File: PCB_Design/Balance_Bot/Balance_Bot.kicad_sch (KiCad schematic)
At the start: 29 parts, among them J1 DC Motor A, J2 DC Motor B, J3 Motor Power, Q1 BSS138, Q2 BSS138, U1 MPU-6050, U2 AP2112K-3.3, U3 DRV8871DDA, U4 DRV8871DDA

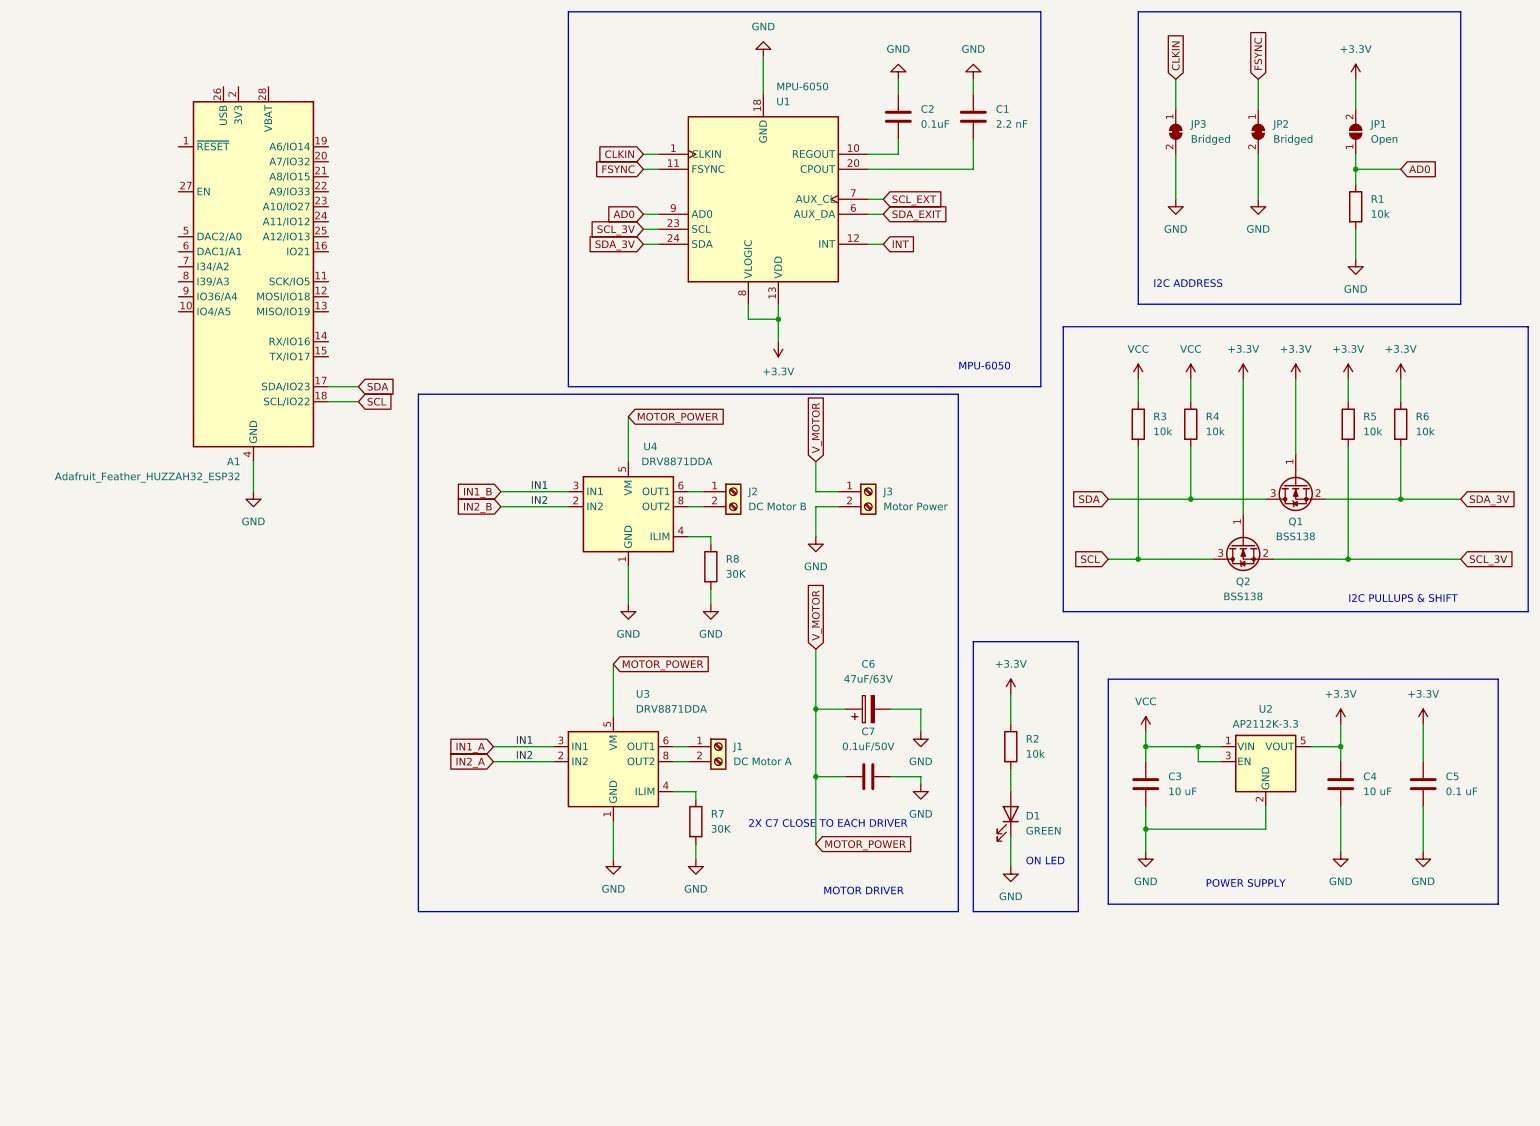
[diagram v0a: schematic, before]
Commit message: board design
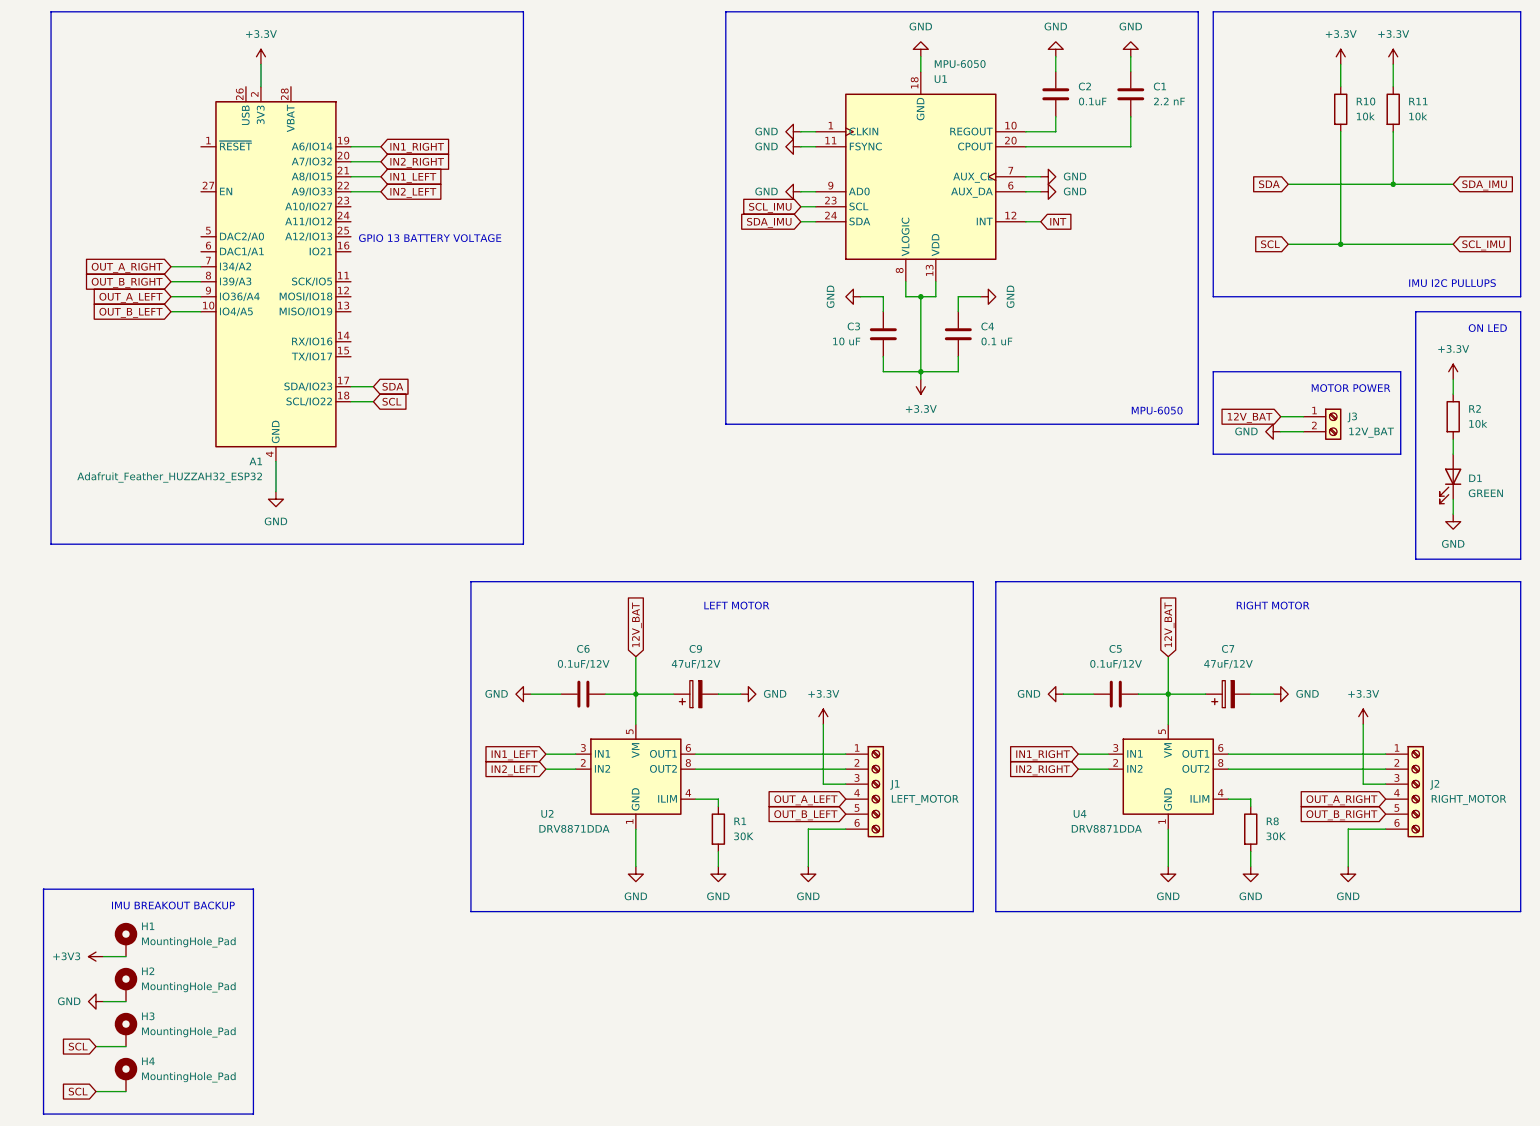
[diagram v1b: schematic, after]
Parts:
- removed C6: 47uF/63V, symbol Device:C_Polarized
- removed C7: 0.1uF/50V, Capacitor_SMD:C_0805_2012Metric, symbol Device:C
- removed J1: DC Motor A, symbol Connector:Screw_Terminal_01x02
- removed J2: DC Motor B, symbol Connector:Screw_Terminal_01x02
- removed JP1: Open, Jumper:SolderJumper-2_P1.3mm_Open_RoundedPad1.0x1.5mm, symbol Jumper:SolderJumper_2_Open
- removed JP2, JP3: Bridged, Jumper:SolderJumper-2_P1.3mm_Bridged_RoundedPad1.0x1.5mm, symbol Jumper:SolderJumper_2_Bridged
- removed Q1, Q2: BSS138, Package_TO_SOT_SMD:SOT-23, symbol Transistor_FET:BSS138
- removed R3, R4, R5, R6: 10k, Resistor_SMD:R_0805_2012Metric, symbol Device:R
- removed R7: 30K, Resistor_SMD:R_0805_2012Metric, symbol Device:R
- removed U2: AP2112K-3.3, Package_TO_SOT_SMD:SOT-23-5, symbol Regulator_Linear:AP2112K-3.3
- removed U3: DRV8871DDA, Package_SO:Texas_HTSOP-8-1EP_3.9x4.9mm_P1.27mm_EP2.95x4.9mm_Mask2.4x3.1mm_ThermalVias, symbol Driver_Motor:DRV8871DDA
- added C6: 0.1uF/12V, Capacitor_SMD:C_0805_2012Metric, symbol Device:C
- added C7, C9: 47uF/12V, symbol Device:C_Polarized
- added H1, H2, H3, H4: MountingHole_Pad, symbol Mechanical:MountingHole_Pad
- added J1: LEFT_MOTOR, TerminalBlock_Phoenix:TerminalBlock_Phoenix_PT-1,5-6-3.5-H_1x06_P3.50mm_Horizontal, symbol Connector:Screw_Terminal_01x06
- added J2: RIGHT_MOTOR, TerminalBlock_Phoenix:TerminalBlock_Phoenix_PT-1,5-6-3.5-H_1x06_P3.50mm_Horizontal, symbol Connector:Screw_Terminal_01x06
- added R10, R11: 10k, Resistor_SMD:R_0805_2012Metric, symbol Device:R
- added U2: DRV8871DDA, Package_SO:Texas_HTSOP-8-1EP_3.9x4.9mm_P1.27mm_EP2.95x4.9mm_Mask2.4x3.1mm_ThermalVias, symbol Driver_Motor:DRV8871DDA
- C4: value 10 uF -> 0.1 uF
- C5: value 0.1 uF -> 0.1uF/12V
- J3: value Motor Power -> 12V_BAT
- R1: value 10k -> 30K
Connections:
- net CLKIN is gone; now on net GND: U1.1 (CLKIN)
- net FSYNC is gone; now on net GND: U1.11 (FSYNC)
- net IN1_A is gone; now on net IN1_RIGHT: U4.3 (IN1)
- net IN2_A is gone; now on net IN2_RIGHT: U4.2 (IN2)
- net SCL_3V is gone; now on net SCL: U1.23 (SCL)
- net SCL_EXT is gone; now on net GND: U1.7 (AUX_CL)
- net SDA_3V is gone; now on net SDA: U1.24 (SDA)
- net SDA_EXIT is gone; now on net GND: U1.6 (AUX_DA)
- net VCC is gone; now on net +3.3V: C3.1
- net +3.3V: now also A1.2 (3V3), J1.3 (Pin_3), J2.3 (Pin_3), R10.1, R11.1; no longer C5.1
- net GND: now also U1.9 (AD0), C6.2, C7.2, C9.2, H2.1, J1.6 (Pin_6), J2.6 (Pin_6), U2.1 (GND), U2.7 (GND), U2.9 (GND)
- net SCL: now also H3.1, H4.1, R10.2
- net SDA: now also R11.2
- net at U4.6 (OUT1): now also J2.1 (Pin_1)
- net at U4.8 (OUT2): now also J2.2 (Pin_2)
- net OUT_B_LEFT: now reaches A1.10 (IO4/A5)
- net OUT_B_LEFT: now also J1.5 (Pin_5)
- net IN1_RIGHT: now reaches A1.19 (A6/IO14)
- net IN2_RIGHT: now reaches A1.20 (A7/IO32)
- net IN1_LEFT: now reaches A1.21 (A8/IO15)
- net IN1_LEFT: now also U2.3 (IN1)
- net IN2_LEFT: now reaches A1.22 (A9/IO33)
- net IN2_LEFT: now also U2.2 (IN2)
- net OUT_A_RIGHT: now reaches A1.7 (I34/A2)
- net OUT_A_RIGHT: now also J2.4 (Pin_4)
- net OUT_B_RIGHT: now reaches A1.8 (I39/A3)
- net OUT_B_RIGHT: now also J2.5 (Pin_5)
- net OUT_A_LEFT: now reaches A1.9 (IO36/A4)
- net OUT_A_LEFT: now also J1.4 (Pin_4)
- net AD0: no longer names the net of R1.1
- net AD0: now also U2.4 (ILIM); no longer U1.9 (AD0)
- net MOTOR_POWER renamed 12V_BAT
- net 12V_BAT: now also C5.1, C6.1, C7.1, C9.1, U2.5 (VM)
- new net: J1.1 (Pin_1), U2.6 (OUT1)
- new net: J1.2 (Pin_2), U2.8 (OUT2)
- new net +3V3: H1.1
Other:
- note added: "GPIO 13 BATTERY VOLTAGE"
- note added: "IMU BREAKOUT BACKUP"
- note added: "IMU I2C PULLUPS"
- note added: "LEFT MOTOR"
- note added: "MOTOR POWER"
- note added: "RIGHT MOTOR"
- note removed: "2X C7 CLOSE TO EACH DRIVER"
- note removed: "I2C ADDRESS"
- note removed: "I2C PULLUPS & SHIFT"
- note removed: "MOTOR DRIVER"
- note removed: "POWER SUPPLY"
- moved on the sheet: A1, C1, C2, D1, J3, R2, R8, U1, U4

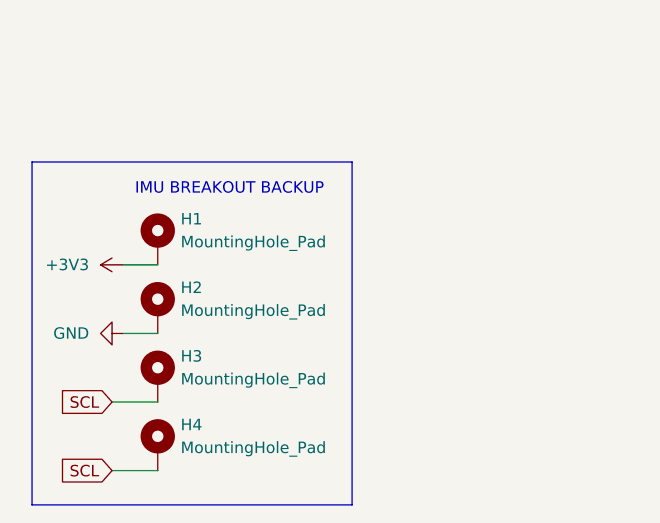
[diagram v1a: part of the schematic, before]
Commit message: board stuff
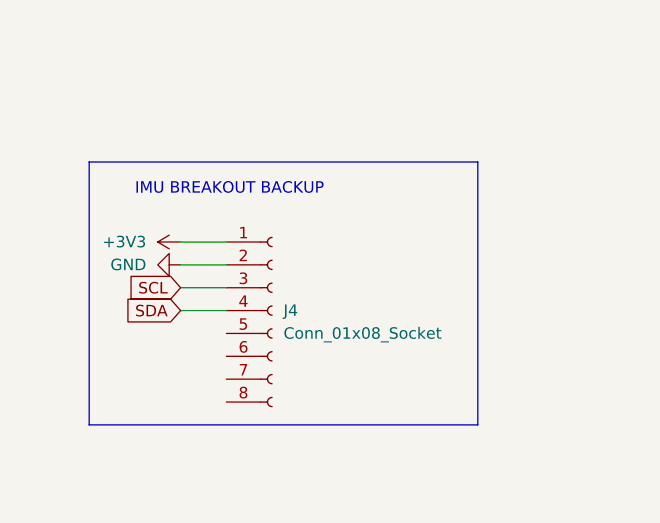
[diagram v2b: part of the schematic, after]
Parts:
- removed H1, H2, H3, H4: MountingHole_Pad, symbol Mechanical:MountingHole_Pad
- added J4: Conn_01x08_Socket, Connector_PinSocket_1.00mm:PinSocket_1x08_P1.00mm_Vertical, symbol Connector:Conn_01x08_Socket
- C7, C9: footprint (none) -> Capacitor_SMD:CP_Elec_5x5.3
- J1, J2: footprint TerminalBlock_Phoenix:TerminalBlock_Phoenix_PT-1,5-6-3.5-H_1x06_P3.50mm_Horizontal -> TerminalBlock_Phoenix:TerminalBlock_Phoenix_MPT-0,5-6-2.54_1x06_P2.54mm_Horizontal
- J3: footprint (none) -> TerminalBlock_Phoenix:TerminalBlock_Phoenix_MPT-0,5-2-2.54_1x02_P2.54mm_Horizontal
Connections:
- net +3V3: now also J4.1 (Pin_1)
- net GND: now also J4.2 (Pin_2)
- net SCL: now also J4.3 (Pin_3)
- net SDA: now also J4.4 (Pin_4)
